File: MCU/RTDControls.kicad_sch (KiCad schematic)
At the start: 2 parts, among them U10 AMC1301DWVR

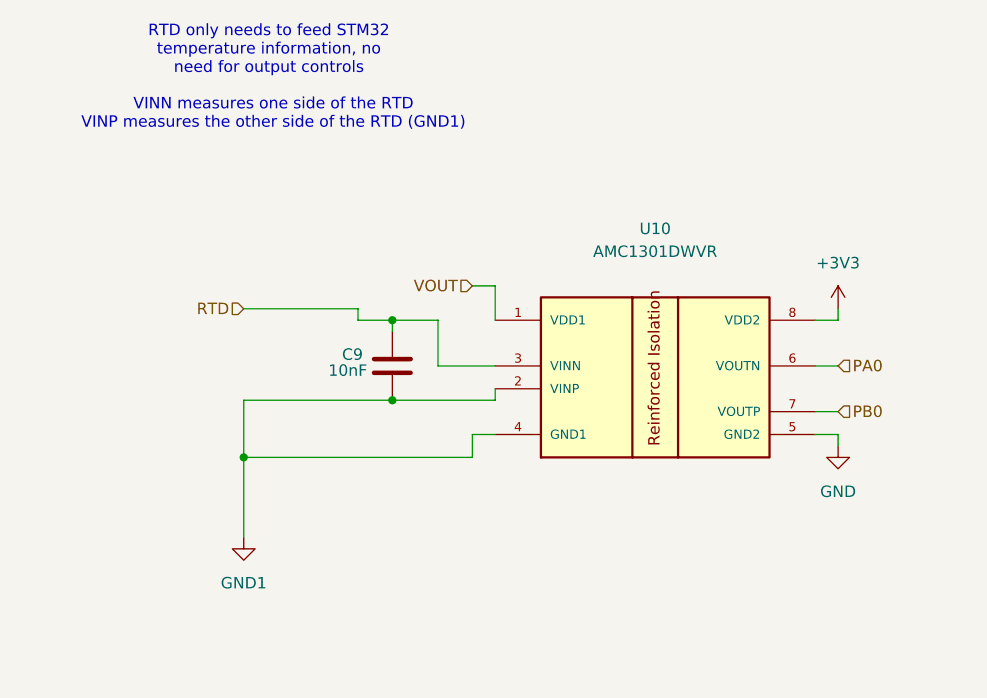
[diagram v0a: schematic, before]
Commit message: Finalized schematic and started layout
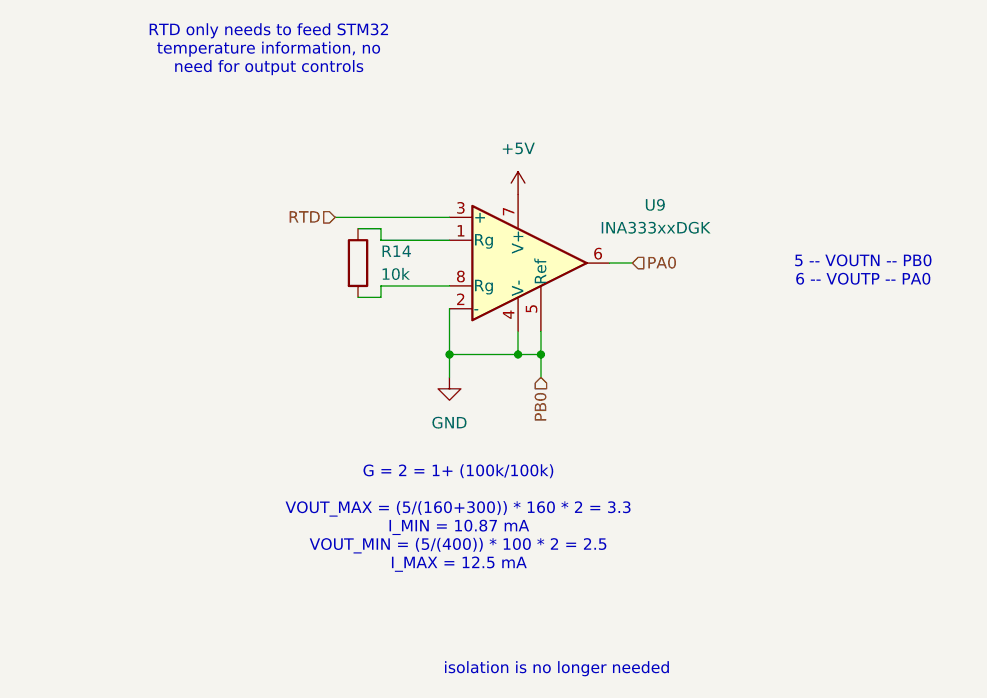
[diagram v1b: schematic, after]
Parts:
- removed C9: 10nF, Capacitor_SMD:C_1206_3216Metric, symbol Device:C
- removed U10: AMC1301DWVR, AMC1301DWVR:SOIC127P1150X280-8N, symbol AMC1301:AMC1301DWVR
- added R14: 10k, Resistor_SMD:R_0603_1608Metric_Pad0.98x0.95mm_HandSolder, symbol Device:R
- added U9: INA333xxDGK, Package_SO:VSSOP-8_3x3mm_P0.65mm, symbol Amplifier_Instrumentation:INA333xxDGK
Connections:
- net GND: now also U9.2 (-), U9.4 (V-), U9.5 (Ref)
- net PA0: now also U9.6
- net RTD: now also U9.3 (+)
- new net: R14.1, U9.1 (Rg)
- new net: R14.2, U9.8 (Rg)
- new net +5V: U9.7 (V+)
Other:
- note added: "5 -- VOUTN -- PB0 6 -- VOUTP -- PA0"
- note added: "G = 2 = 1+ (100k/100k) VOUT_MAX = (5/(160+300)) * 160 * 2 = 3.3 I_MIN = 10.87 mA VOUT_MIN = (5/(400)) * 100 * 2 = 2.5 I_MAX = 12.5 mA"
- note added: "isolation is no longer needed"
- note removed: "VINN measures one side of the RTD VINP measures the other side of the RTD (GND1)"
